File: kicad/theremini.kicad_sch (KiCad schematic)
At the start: 30 parts, among them SW1 K2-1157SP-I4SW-04, U1 NAU88C22YG, U10 TPS63051RMWR, U2 VL53L0CXV0DH/1, U4 VL53L0CXV0DH/1, U5 KLJ-01304T-08R07W, U6 PJ-327C-4A, U7 STM32L432KBU6TR, U8 YTS1C0033BBG01, U9 TYPE-C16PIN, X1 OT32258MJBA4SL

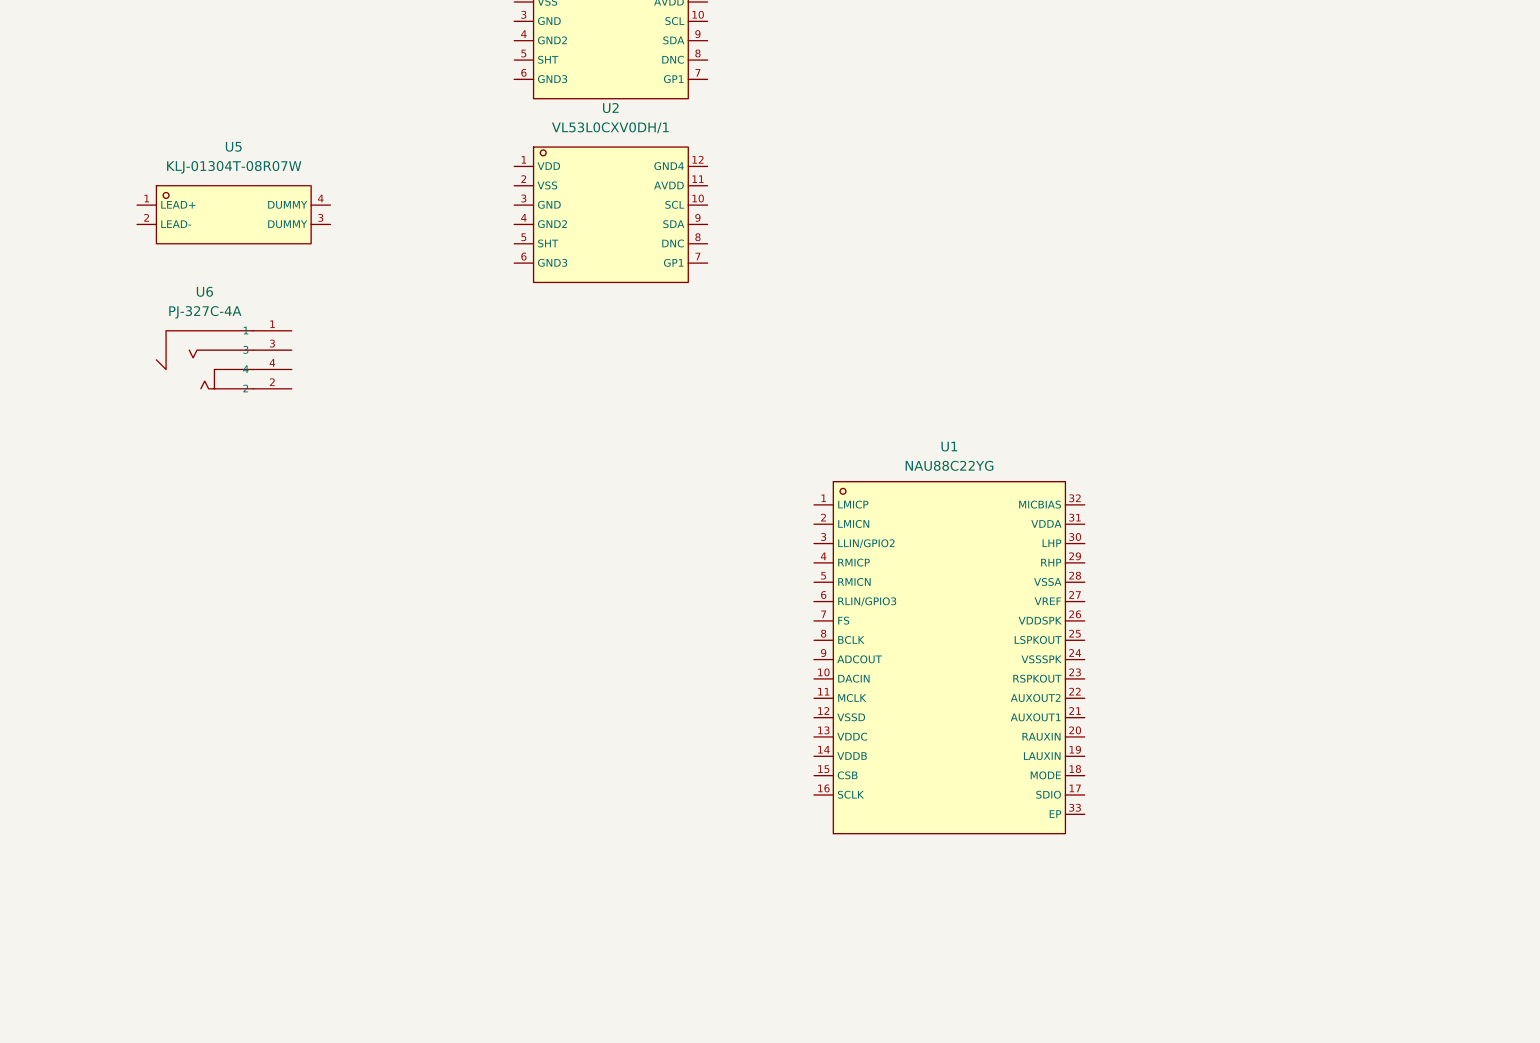
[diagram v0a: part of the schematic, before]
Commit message: quick quick quiiick
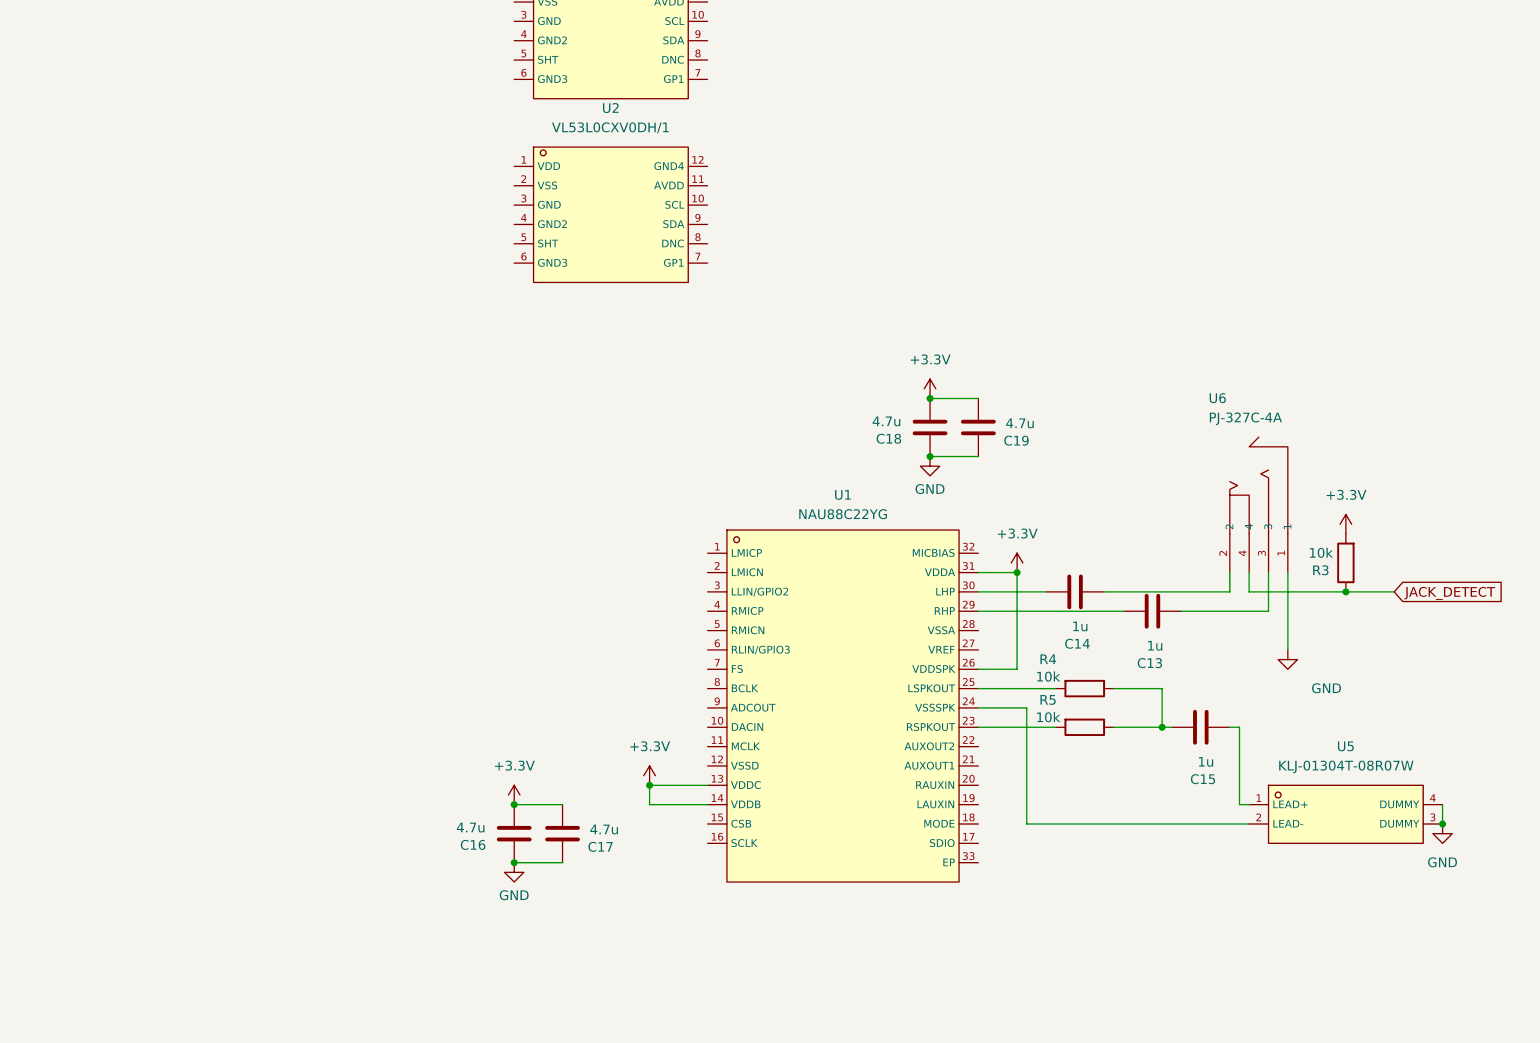
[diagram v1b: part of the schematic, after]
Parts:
- added C13, C14, C15: 1u, Capacitor_SMD:C_0402_1005Metric, symbol Device:C
- added C16, C17, C18, C19: 4.7u, Capacitor_SMD:C_0402_1005Metric, symbol Device:C
- added R3, R4, R5: 10k, Resistor_SMD:R_0201_0603Metric, symbol Device:R
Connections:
- net +3.3V: now also U1.13 (VDDC), U1.14 (VDDB), U1.26 (VDDSPK), U1.31 (VDDA), C16.1, C17.1, C18.1, C19.1, R3.2
- net GND: now also U5.3 (DUMMY), U5.4 (DUMMY), U6.1, C16.2, C17.2, C18.2, C19.2
- net at U5.1 (LEAD+): now also C15.2
- net at U5.2 (LEAD-): now also U1.24 (VSSSPK)
- net at U6.2: now also C14.2
- net at U6.3: now also C13.1
- net JACK_DETECT: now reaches U6.4
- net JACK_DETECT: now also R3.1
- net at U1.23 (RSPKOUT): now also R5.2
- net at U1.25 (LSPKOUT): now also R4.2
- net at U1.29 (RHP): now also C13.2
- net at U1.30 (LHP): now also C14.1
- new net: C15.1, R4.1, R5.1
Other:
- moved on the sheet: U1, U5, U6
